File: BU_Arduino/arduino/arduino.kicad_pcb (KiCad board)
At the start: 2 copper layers, 89.7 x 55.1 mm, 52 parts, among them CON1 ICSP, J1 USB_A, J2 Barrel_Jack, J3 Power, J4 Digital, J5 Digital, J6 Analog, Q1 FDN340P, SW1 SW_Push_Dual, U1 NCP1117-12_TO252, U2 ATMEGA32U4-AU, U3 LMV358, U4 LP2985-3.3, Y1 16MHz

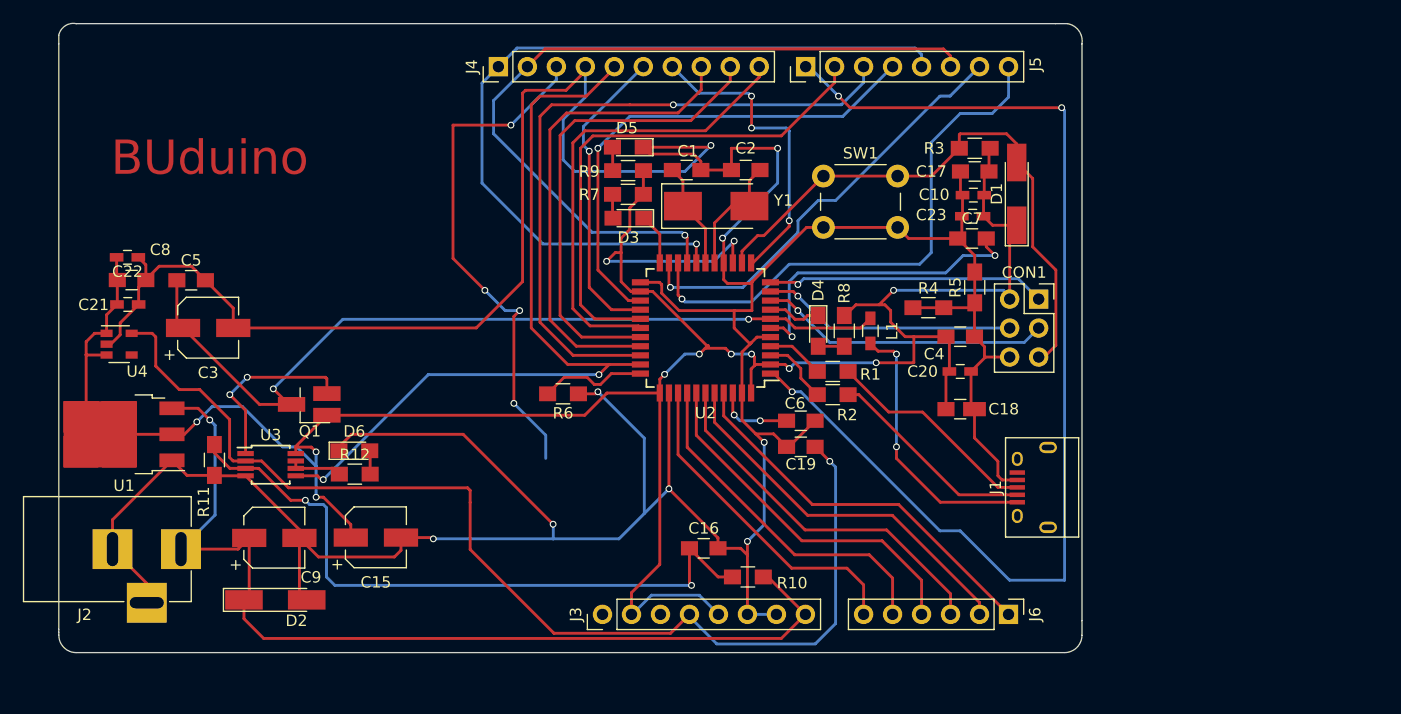
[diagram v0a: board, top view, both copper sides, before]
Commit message: Updated few files
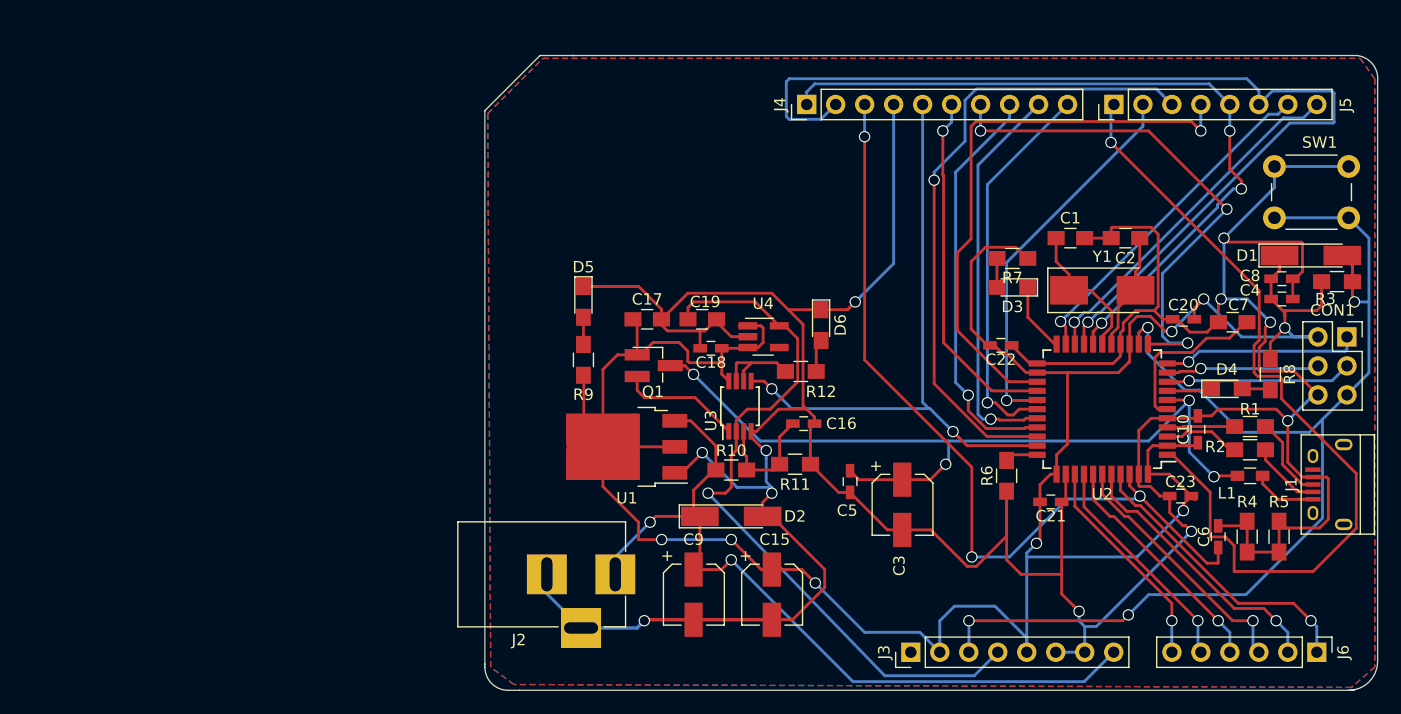
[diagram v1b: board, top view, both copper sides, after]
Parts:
- C16, C18, C4, C5, C6, C8: footprint Capacitors_SMD:C_0805_HandSoldering -> Capacitors_SMD:C_0603_HandSoldering
- moved C8 100.8 mm to (204.0, 100.6)
- moved C21 82.7 mm to (183.7, 120.1)
- moved C22 76.9 mm to (179.3, 106.4)
- moved C3 62.8 mm to (170.7, 120.4), turned to 270 degrees
- moved C5 60.4 mm to (166.1, 118.4), turned to 270 degrees
- moved U4 56.4 mm to (158.5, 105.7)
- moved R11 50.9 mm to (161.3, 116.8), turned to 0 degrees
- moved SW1 46.2 mm to (209.8, 95.2), turned to 180 degrees
- moved U1 44.1 mm to (146.6, 115.3)
- moved D6 42.4 mm to (163.6, 104.6), turned to 270 degrees
- moved U3 41.4 mm to (156.5, 111.8), turned to 90 degrees
- moved D2 40.6 mm to (155.7, 121.4)
- moved R12 40.1 mm to (161.8, 108.7)
- moved R6 39.5 mm to (179.8, 117.9), turned to 90 degrees
- moved J2 38.1 mm to (145.5, 126.5)
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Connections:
- C6 pad 1: Net-(C6-Pad1) -> /AREF
- CON1 pad 5: Net-(CON1-Pad5) -> /RST
- D1 pad 2: Net-(CON1-Pad5) -> /RST
- J3 pad 3: /RESET -> /RST
- R3 pad 2: Net-(CON1-Pad5) -> /RST
- SW1 pad 1: Net-(CON1-Pad5) -> /RST
- U2 pad 13: Net-(CON1-Pad5) -> /RST
- U2 pad 42: Net-(C6-Pad1) -> /AREF
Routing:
- net /RST: track 0.00 -> 104.0 mm, vias 0 -> 4
- net Net-(CON1-Pad5): track 51.4 -> 0.00 mm
- net Net-(C16-Pad1): track 59.0 -> 10.6 mm, vias 2 -> 0
- net +3V3: track 97.9 -> 64.1 mm
- net /AREF: track 45.6 -> 73.4 mm, vias 4 -> 3
- net /D7: track 98.7 -> 73.6 mm, vias 3 -> 1
- net GND: track 373.9 -> 349.8 mm, vias 9 -> 11
- net /D2/SDA: track 69.0 -> 91.9 mm
- net /IO11: track 27.3 -> 46.2 mm
- net Net-(J1-Pad1): track 24.0 -> 5.67 mm, vias 2 -> 0
- net /VIN: track 87.7 -> 70.2 mm, vias 1 -> 2
- net /D0/RX: track 47.8 -> 31.1 mm
- net /IO13: track 71.0 -> 54.3 mm
- net Net-(C7-Pad2): track 27.9 -> 14.8 mm, vias 2 -> 0
- net Net-(J1-Pad2): track 18.5 -> 6.22 mm
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- added copper zone on B.Cu, net GND
- added copper zone on F.Cu, net GND
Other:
- board size 89.7 x 55.1 mm -> 78.2 x 55.6 mm
